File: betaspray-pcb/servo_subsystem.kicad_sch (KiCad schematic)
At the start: 17 parts, among them J11 Conn_01x03_Pin, J12 Conn_01x03_Pin, J13 Conn_01x03_Pin, J14 Conn_01x03_Pin, J15 Conn_01x03_Pin, J16 Conn_01x03_Pin, J17 Conn_01x03_Pin, J18 Conn_01x03_Pin, J2 Conn_01x02, J3 Conn_01x02, J4 Conn_01x02, J5 Conn_01x02, Q1 AO3400A

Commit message: Ver0, pls'
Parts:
- C10, C11: footprint (none) -> Capacitor_THT:CP_Radial_D16.0mm_P7.50mm
- R7, R8: footprint (none) -> Resistor_SMD:R_0805_2012Metric_Pad1.20x1.40mm_HandSolder
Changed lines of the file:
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@@
 			)
 		)
-		(property "Footprint" ""
+		(property "Footprint" "Resistor_SMD:R_0805_2012Metric_Pad1.20x1.40mm_HandSolder"
 			(at 154.178 113.03 90)
 			(effects
@@
 			)
 		)
-		(property "Footprint" ""
+		(property "Footprint" "Capacitor_THT:CP_Radial_D16.0mm_P7.50mm"
 			(at 56.8452 129.54 0)
 			(effects
@@
 			)
 		)
-		(property "Footprint" ""
+		(property "Footprint" "Capacitor_THT:CP_Radial_D16.0mm_P7.50mm"
 			(at 35.2552 129.54 0)
 			(effects
@@
 			)
 		)
-		(property "Footprint" ""
+		(property "Footprint" "Resistor_SMD:R_0805_2012Metric_Pad1.20x1.40mm_HandSolder"
 			(at 144.78 107.188 90)
 			(effects

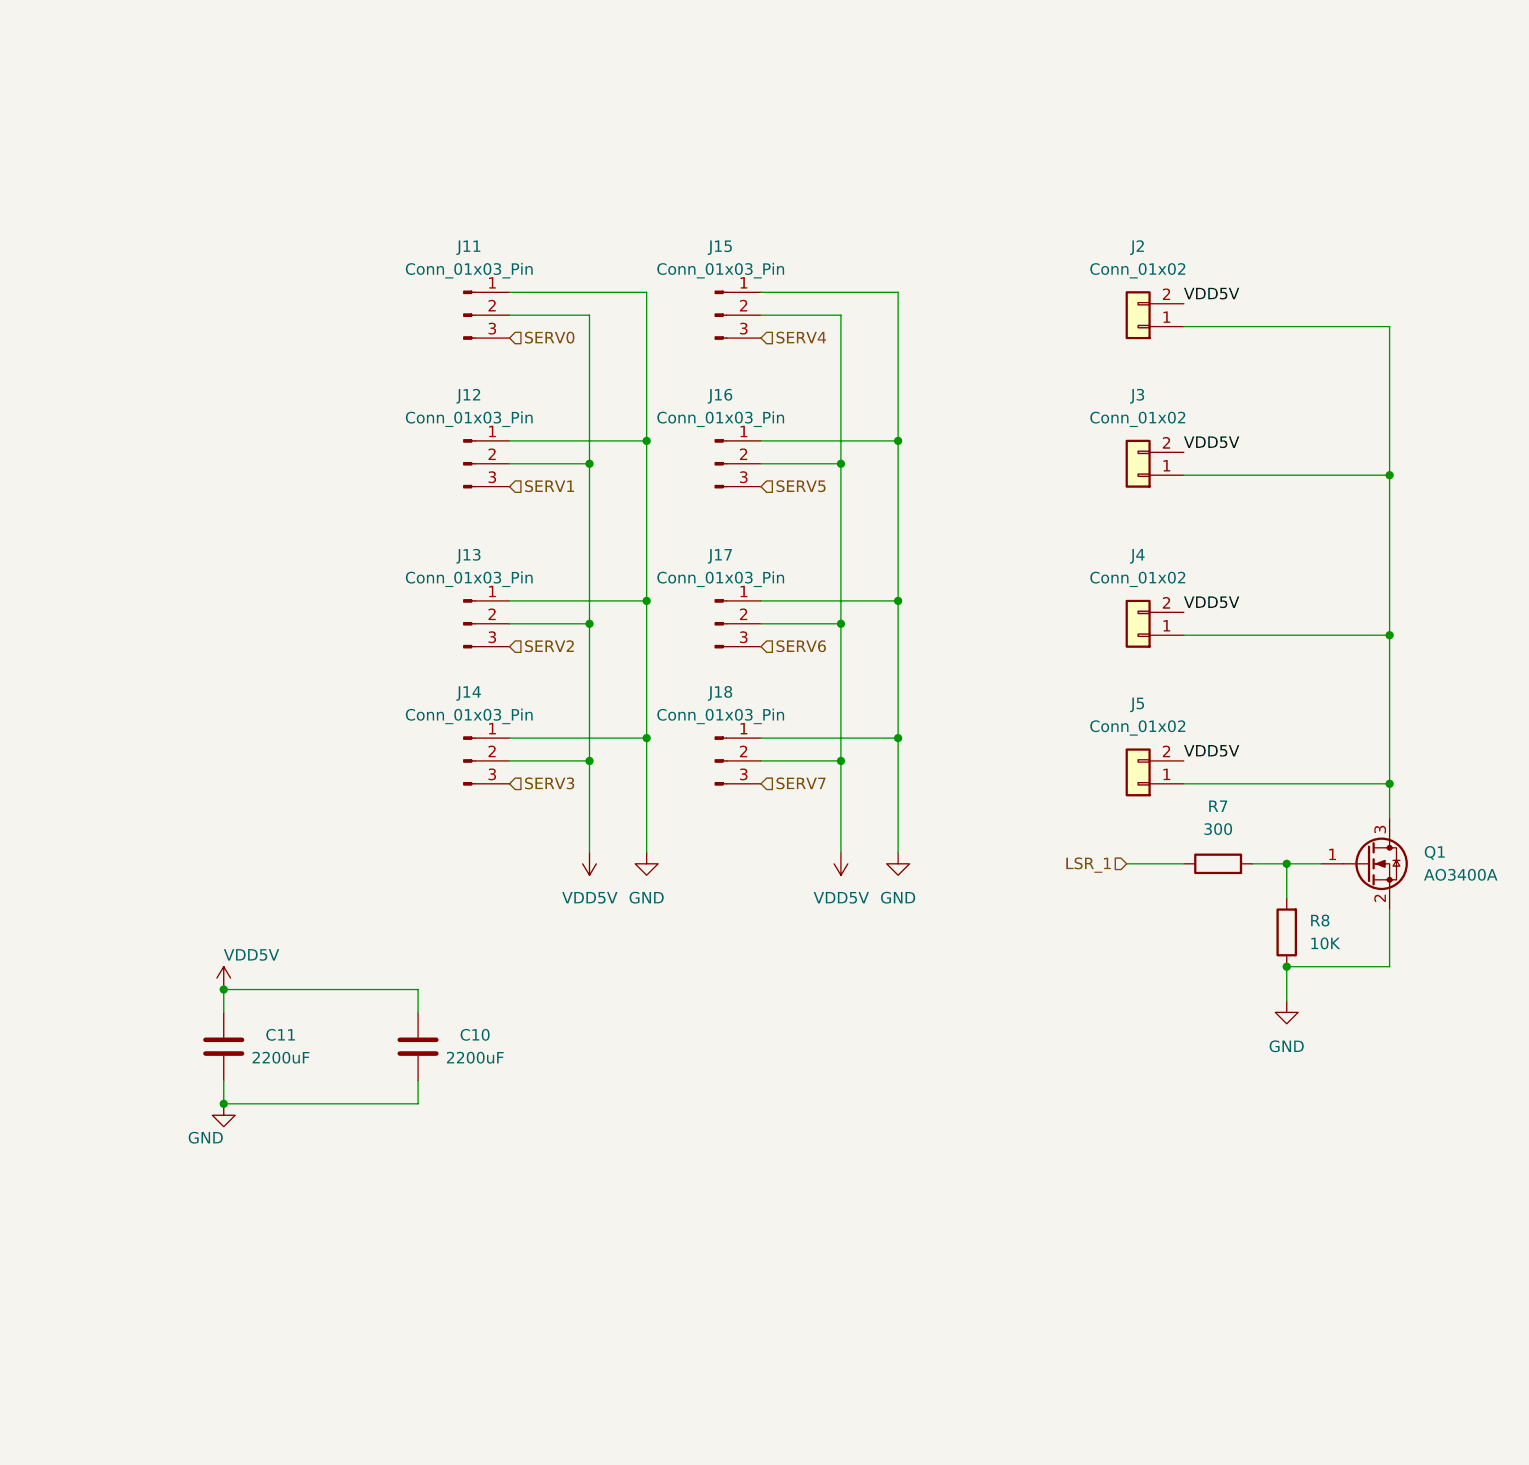
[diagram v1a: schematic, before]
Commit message: Tweak pcb slightly
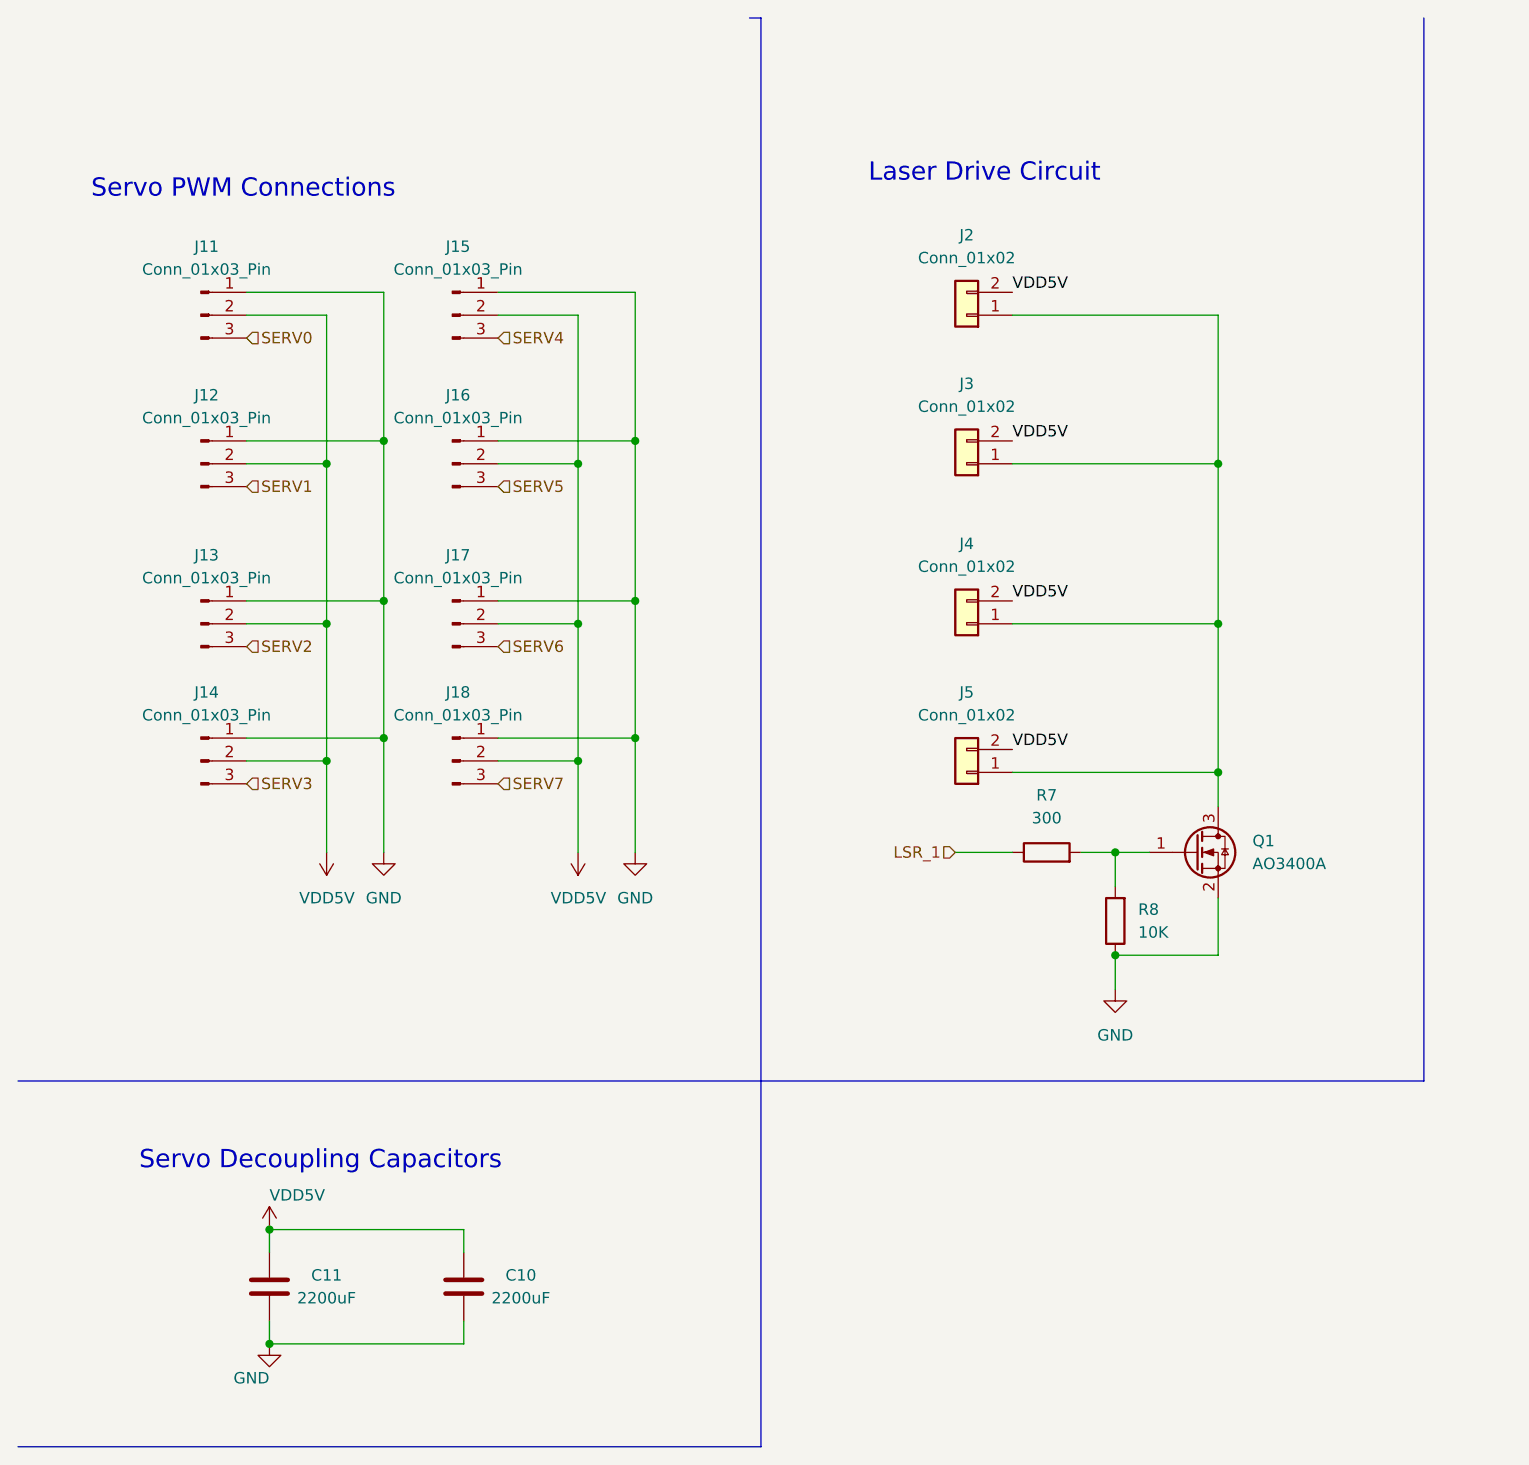
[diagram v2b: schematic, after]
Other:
- note added: "Laser Drive Circuit"
- note added: "Servo Decoupling Capacitors"
- note added: "Servo PWM Connections"
- moved on the sheet: C10, C11, J11, J12, J13, J14, J15, J16, J17, J18, J2, J3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
